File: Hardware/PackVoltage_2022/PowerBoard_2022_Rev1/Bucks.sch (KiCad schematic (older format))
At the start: 80 parts, among them U10 OKI-78SR-12_1.0-W36-C, U11 OKI-78SR-12_1.0-W36-C, U12 OKI-78SR-12_1.0-W36-C, U13 OKI-78SR-12_1.0-W36-C, U14 OKI-78SR-12_1.0-W36-C, U15 OKI-78SR-12_1.0-W36-C, U16 OKI-78SR-12_1.0-W36-C, U17 OKI-78SR-12_1.0-W36-C, U55 OKI-78SR-12_1.0-W36-C, U7 OKI-78SR-5_1.5-W36-C, U8 OKI-78SR-3.3_1.5-W36-C, U9 OKI-78SR-12_1.0-W36-C

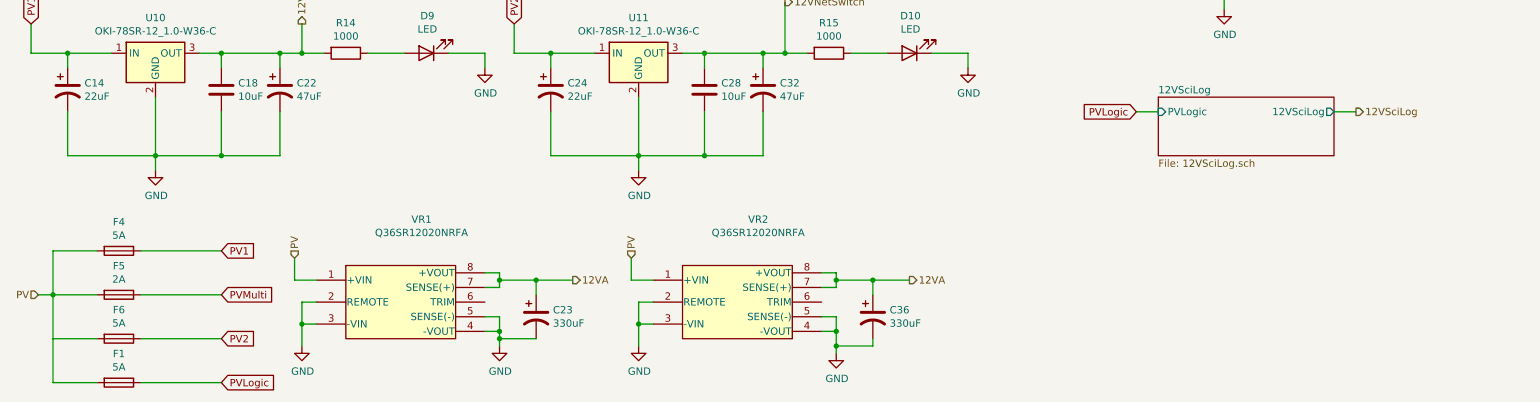
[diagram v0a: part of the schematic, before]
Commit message: Actuation shit
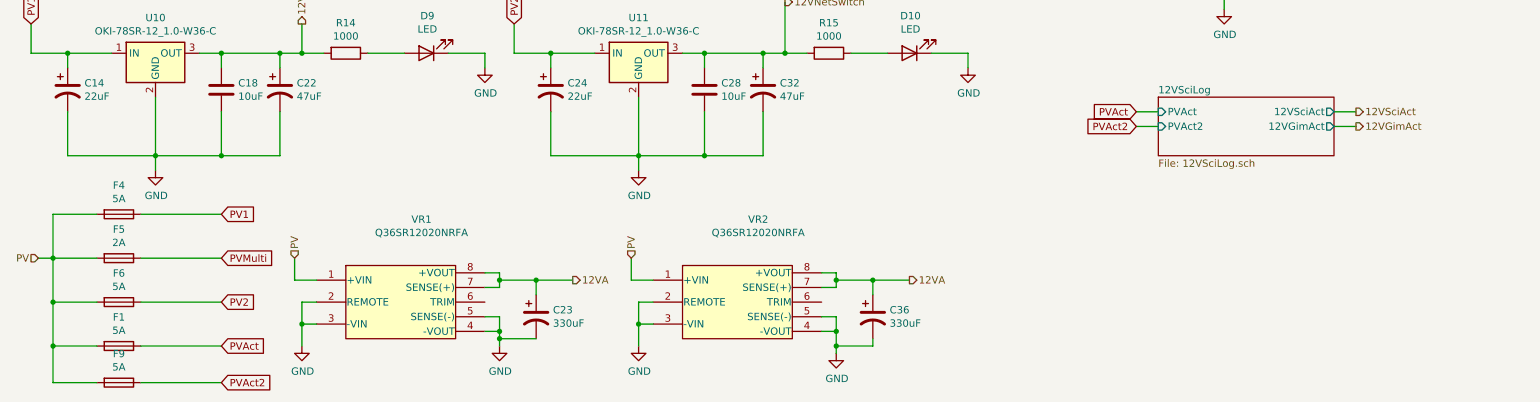
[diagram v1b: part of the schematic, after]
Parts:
- added F9: 5A, Fuse:Fuse_0603_1608Metric_Pad1.05x0.95mm_HandSolder, symbol Device:Fuse
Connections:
- net PV: now also F9.2
- net PVLogic renamed PVAct
- new net PVAct2: F9.1
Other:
- moved on the sheet: F1, F4, F5, F6
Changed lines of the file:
@@
 Wire Wire Line
 	6000 3750 6150 3750
-Text HLabel 750  7000 0    50   Input ~ 0
+Text HLabel 750  6750 0    50   Input ~ 0
 PV
 $Comp
 L Device:Fuse F4
 U 1 1 61DCC65E
-P 1300 6700
-F 0 "F4" V 1103 6700 50  0000 C CNN
-F 1 "5A" V 1194 6700 50  0000 C CNN
-F 2 "Fuse:Fuse_0603_1608Metric_Pad1.05x0.95mm_HandSolder" V 1230 6700 50  0001 C CNN
-F 3 "~" H 1300 6700 50  0001 C CNN
-	1    1300 6700
+P 1300 6450
+F 0 "F4" V 1103 6450 50  0000 C CNN
+F 1 "5A" V 1194 6450 50  0000 C CNN
+F 2 "Fuse:Fuse_0603_1608Metric_Pad1.05x0.95mm_HandSolder" V 1230 6450 50  0001 C CNN
+F 3 "~" H 1300 6450 50  0001 C CNN
+	1    1300 6450
 	0    1    1    0
 $EndComp
@@
 L Device:Fuse F6
 U 1 1 61DCD94F
-P 1300 7300
-F 0 "F6" V 1103 7300 50  0000 C CNN
-F 1 "5A" V 1194 7300 50  0000 C CNN
-F 2 "Fuse:Fuse_0603_1608Metric_Pad1.05x0.95mm_HandSolder" V 1230 7300 50  0001 C CNN
-F 3 "~" H 1300 7300 50  0001 C CNN
-	1    1300 7300
-	0    1    1    0
-$EndComp
-Text GLabel 2000 6700 2    50   Input ~ 0
+P 1300 7050
+F 0 "F6" V 1103 7050 50  0000 C CNN
+F 1 "5A" V 1194 7050 50  0000 C CNN
+F 2 "Fuse:Fuse_0603_1608Metric_Pad1.05x0.95mm_HandSolder" V 1230 7050 50  0001 C CNN
+F 3 "~" H 1300 7050 50  0001 C CNN
+	1    1300 7050
+	0    1    1    0
+$EndComp
+Text GLabel 2000 6450 2    50   Input ~ 0
 PV1
-Text GLabel 2000 7300 2    50   Input ~ 0
+Text GLabel 2000 7050 2    50   Input ~ 0
 PV2
 Wire Wire Line
-	1450 6700 2000 6700
-Wire Wire Line
-	1450 7300 2000 7300
-Wire Wire Line
-	1150 6700 850  6700
-Wire Wire Line
-	1150 7300 850  7300
-Wire Wire Line
-	850  6700 850  7000
+	1450 6450 2000 6450
+Wire Wire Line
+	1450 7050 2000 7050
+Wire Wire Line
+	1150 6450 850  6450
+Wire Wire Line
+	1150 7050 850  7050
+Wire Wire Line
+	850  6450 850  6750
 Text GLabel 700  3450 1    50   Input ~ 0
 PV1
@@
 L Device:Fuse F5
 U 1 1 61E23D5F
-P 1300 7000
-F 0 "F5" V 1103 7000 50  0000 C CNN
-F 1 "2A" V 1194 7000 50  0000 C CNN
-F 2 "Fuse:Fuse_0603_1608Metric_Pad1.05x0.95mm_HandSolder" V 1230 7000 50  0001 C CNN
-F 3 "~" H 1300 7000 50  0001 C CNN
-	1    1300 7000
-	0    1    1    0
-$EndComp
-Wire Wire Line
-	1150 7000 850  7000
-Connection ~ 850  7000
-Wire Wire Line
-	850  7000 850  7300
-Wire Wire Line
-	750  7000 850  7000
+P 1300 6750
+F 0 "F5" V 1103 6750 50  0000 C CNN
+F 1 "2A" V 1194 6750 50  0000 C CNN
+F 2 "Fuse:Fuse_0603_1608Metric_Pad1.05x0.95mm_HandSolder" V 1230 6750 50  0001 C CNN
+F 3 "~" H 1300 6750 50  0001 C CNN
+	1    1300 6750
+	0    1    1    0
+$EndComp
+Wire Wire Line
+	1150 6750 850  6750
+Connection ~ 850  6750
+Wire Wire Line
+	850  6750 850  7050
+Wire Wire Line
+	750  6750 850  6750
 $Comp
 L PowerBoard_2022_Rev1-rescue:OKI-78SR-12_1.0-W36-C-Converter_DCDC U10
@@
 Text GLabel 4000 5150 1    50   Input ~ 0
 PV2
-Text GLabel 2000 7000 2    50   Input ~ 0
+Text GLabel 2000 6750 2    50   Input ~ 0
 PVMulti
 Wire Wire Line
-	2000 7000 1450 7000
+	2000 6750 1450 6750
 Wire Wire Line
 	6050 650  6050 1000
@@
 F0 "12VSciLog" 50
 F1 "12VSciLog.sch" 50
-F2 "12VSciLog" O R 9600 5750 50
-F3 "PVLogic" I L 8400 5750 50
+F2 "12VSciAct" O R 9600 5750 50
+F3 "PVAct" I L 8400 5750 50
+F4 "12VGimAct" O R 9600 5850 50
+F5 "PVAct2" I L 8400 5850 50
 $EndSheet
 $Comp
 L Device:Fuse F1
 U 1 1 61E9458E
+P 1300 7350
+F 0 "F1" V 1103 7350 50  0000 C CNN
+F 1 "5A" V 1194 7350 50  0000 C CNN
+F 2 "Fuse:Fuse_0603_1608Metric_Pad1.05x0.95mm_HandSolder" V 1230 7350 50  0001 C CNN
+F 3 "~" H 1300 7350 50  0001 C CNN
+	1    1300 7350
+	0    1    1    0
+$EndComp
+Text GLabel 2000 7350 2    50   Input ~ 0
+PVAct
+Wire Wire Line
+	1450 7350 2000 7350
+Text GLabel 8250 5750 0    50   Input ~ 0
+PVAct
+Wire Wire Line
+	8250 5750 8400 5750
+Text HLabel 9750 5750 2    50   Output ~ 0
+12VSciAct
+Wire Wire Line
+	9600 5750 9750 5750
+Connection ~ 850  7050
+$Comp
+L Device:Fuse F9
+U 1 1 6197848B
 P 1300 7600
-F 0 "F1" V 1103 7600 50  0000 C CNN
+F 0 "F9" V 1103 7600 50  0000 C CNN
 F 1 "5A" V 1194 7600 50  0000 C CNN
 F 2 "Fuse:Fuse_0603_1608Metric_Pad1.05x0.95mm_HandSolder" V 1230 7600 50  0001 C CNN
@@
 $EndComp
 Text GLabel 2000 7600 2    50   Input ~ 0
-PVLogic
+PVAct2
 Wire Wire Line
 	1450 7600 2000 7600
@@
 	1150 7600 850  7600
 Wire Wire Line
-	850  7300 850  7600
-Text GLabel 8250 5750 0    50   Input ~ 0
-PVLogic
-Wire Wire Line
-	8250 5750 8400 5750
-Text HLabel 9750 5750 2    50   Output ~ 0
-12VSciLog
-Wire Wire Line
-	9600 5750 9750 5750
+	850  7050 850  7350
+Wire Wire Line
+	1150 7350 850  7350
+Connection ~ 850  7350
+Wire Wire Line
+	850  7350 850  7600
+Text GLabel 8250 5850 0    50   Input ~ 0
+PVAct2
+Wire Wire Line
+	8250 5850 8400 5850
+Wire Wire Line
+	9600 5850 9750 5850
+Text HLabel 9750 5850 2    50   Output ~ 0
+12VGimAct
 $EndSCHEMATC
